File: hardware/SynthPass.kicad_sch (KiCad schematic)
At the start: 19 parts, among them P1 USB_C_Plug_USB2.0, SW1 SW_Push, U2 CH572D, Y2 32MHz

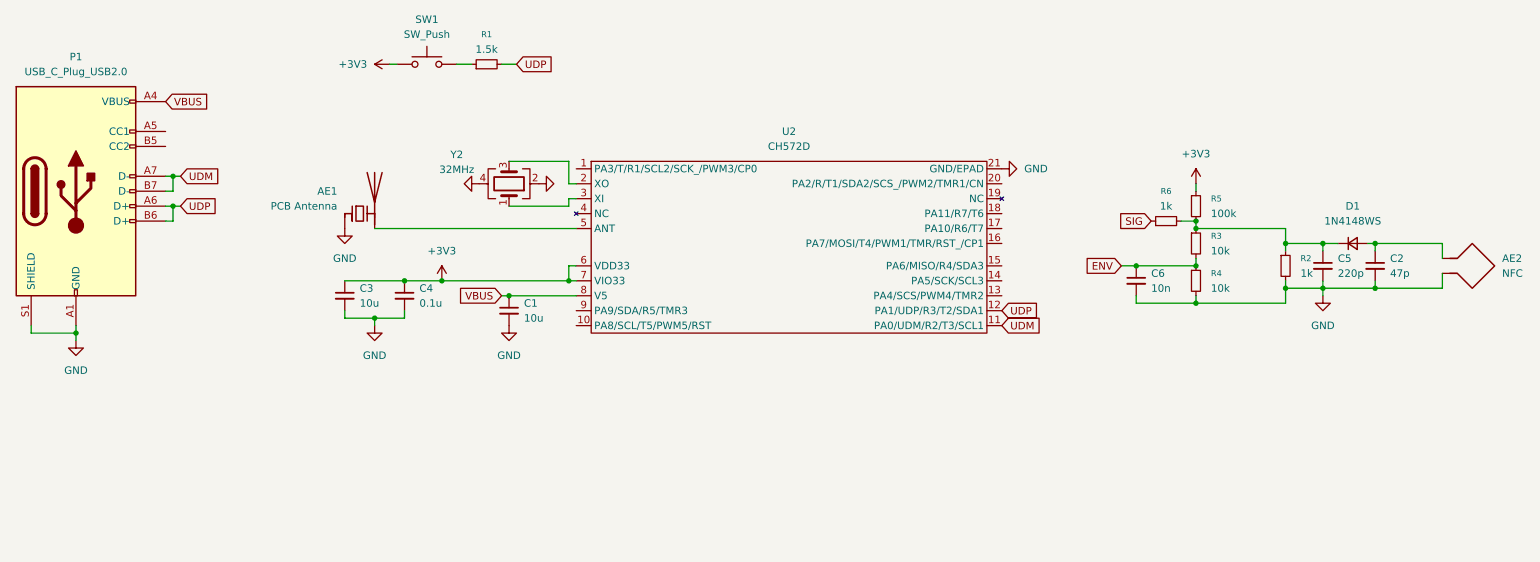
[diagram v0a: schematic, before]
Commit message: Finalize hardware design, pending pinout confirmation
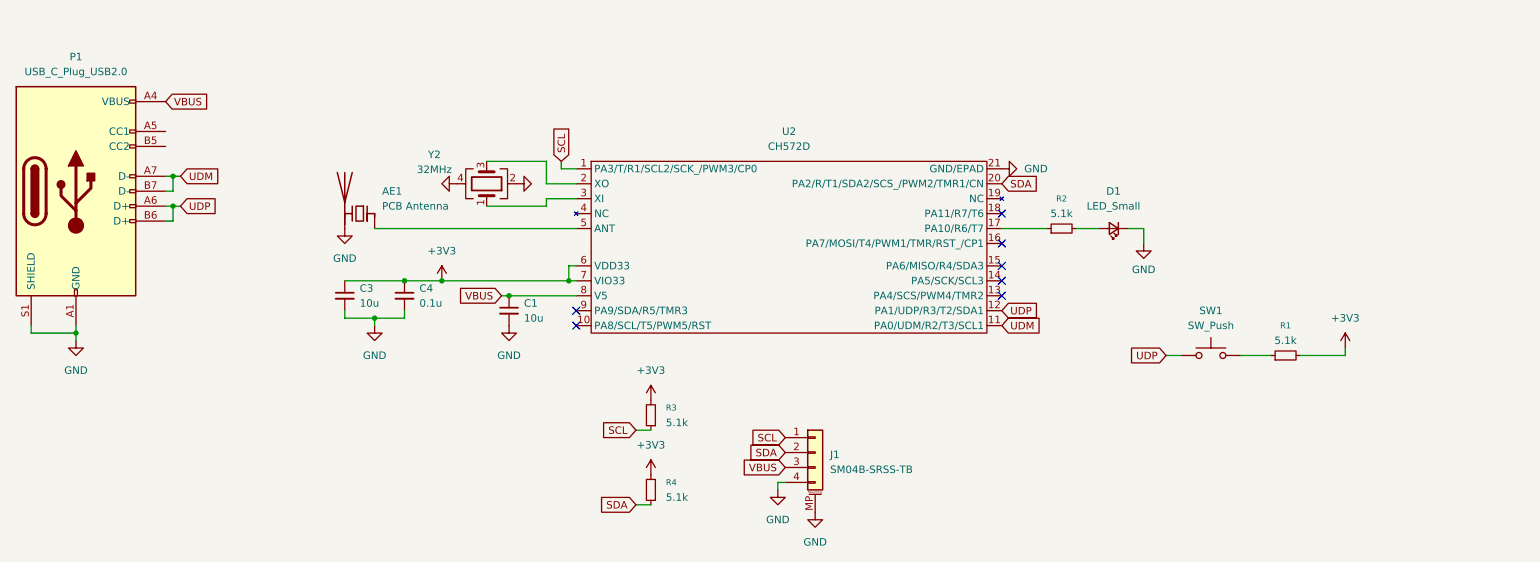
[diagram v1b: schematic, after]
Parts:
- removed AE2: NFC, NFC_Antenna:Antenna_21x17_6T, symbol Device:Antenna_Loop
- removed C2: 47p, Capacitor_SMD:C_0402_1005Metric, symbol Device:C_Small
- removed C5: 220p, Capacitor_SMD:C_0402_1005Metric, symbol Device:C_Small
- removed C6: 10n, Capacitor_SMD:C_0402_1005Metric, symbol Device:C_Small
- removed D1: 1N4148WS, Diode_SMD:D_SOD-323, symbol Device:D_Small
- removed R5: 100k, Resistor_SMD:R_0402_1005Metric, symbol Device:R_Small
- removed R6: 1k, Resistor_SMD:R_0402_1005Metric, symbol Device:R_Small
- added D1: LED_Small, LED_SMD:LED_0603_1608Metric, symbol Device:LED_Small
- added J1: SM04B-SRSS-TB, Connector_JST:JST_SH_SM04B-SRSS-TB_1x04-1MP_P1.00mm_Horizontal, symbol Connector_Generic_MountingPin:Conn_01x04_MountingPin
- P1: footprint PCM_PCB_USBC:PCBTypeC_14P -> Connector_USB:USB_C_Receptacle_G-Switch_GT-USB-7010ASV
- R1: value 1.5k -> 5.1k
- R2: value 1k -> 5.1k
- R3, R4: value 10k -> 5.1k
- SW1: footprint Button_Switch_SMD:SW_Push_1P1T_XKB_TS-1187A -> Button_Switch_SMD:SW_SPST_TS-1088-xR020; LCSC C318884 -> (none)
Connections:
- net +3V3: now also R1.2, R3.2, R4.2; no longer SW1.1
- net GND: now also AE1.2 (PCB_Trace), D1.1 (K), J1.4 (Pin_4), J1.MP (MountPin); no longer AE1.1 (FEED), R2.2, R4.2
- net UDP: now also SW1.1; no longer R1.2
- net VBUS: now also J1.3 (Pin_3)
- net at R2.1: now also U2.17 (PA10/R6/T7); no longer R3.1
- net SCL: now reaches U2.1 (PA3/T/R1/SCL2/SCK_/PWM3/CP0)
- net SCL: now also R3.1, J1.1 (Pin_1)
- net SDA: now reaches U2.20 (PA2/R/T1/SDA2/SCS_/PWM2/TMR1/CN)
- net SDA: now also R4.1, J1.2 (Pin_2)
- net at U2.5 (ANT): now also AE1.1 (FEED); no longer AE1.2 (PCB_Trace)
- removed net ENV: R3.2, R4.1
- new net: D1.2 (A), R2.2
- no-connect marks 0 -> 7
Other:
- moved on the sheet: AE1, Y2
